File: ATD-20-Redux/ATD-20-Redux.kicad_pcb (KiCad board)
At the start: 2 copper layers, 21.8 x 56.6 mm, 5 parts, among them J1 RTC Pins, U1 DS1315, Y1 32.768 KHz

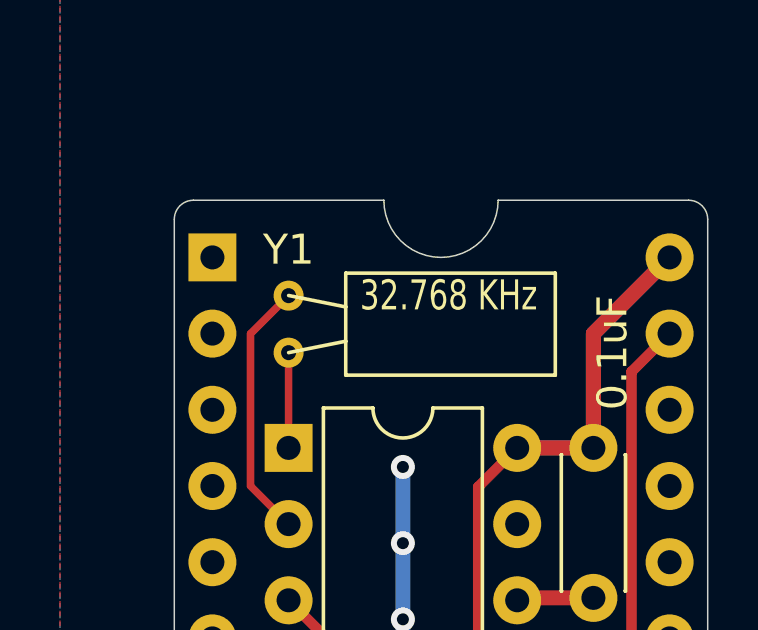
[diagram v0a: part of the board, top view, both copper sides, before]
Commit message: Minor changes to ATD-20-Redux.
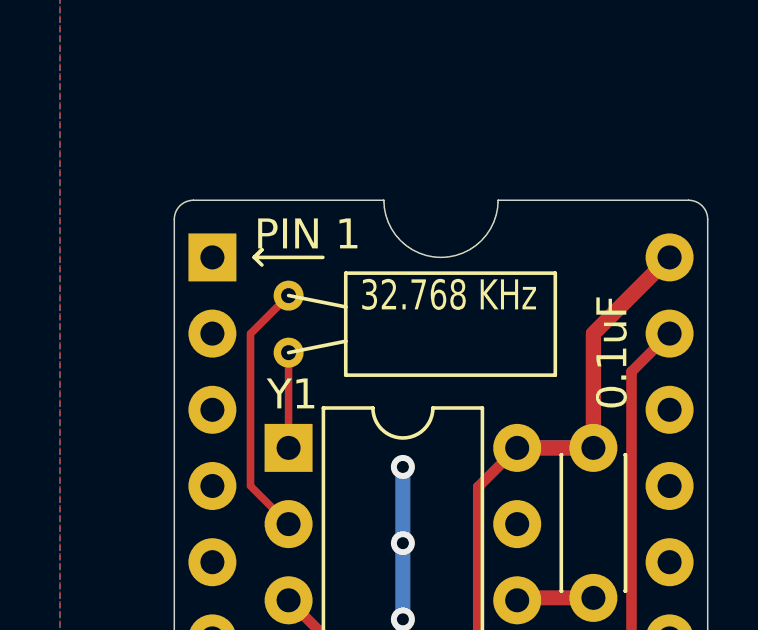
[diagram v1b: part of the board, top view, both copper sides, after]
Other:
- board text added: "PIN 1"
